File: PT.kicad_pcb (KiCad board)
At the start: 4 copper layers, 67 x 68 mm, 111 parts, among them J1 Conn_02x05_Odd_Even, J10 Conn_02x01, J11 Screw_Terminal_01x02, J2 USB_C_Receptacle_USB2.0_16P, J3 Conn_02x01, J4 Conn_02x01, J5 Screw_Terminal_01x05, J6 RJ45_Hanrun_HR911105A_Horizon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, J7 Conn_02x01, J8 Conn_02x01, J9 Conn_02x01, SW1 SKRPANE010, U1 USBLC6-2SC6, U2 STM32H563RIVx, U3 AP2112K-3.3, U4 TJA1042T-3, U5 LAN8742A, U6 ADS131A04, Y1 25 MHz, Y2 25 MHz, Y3 16.384 MHz

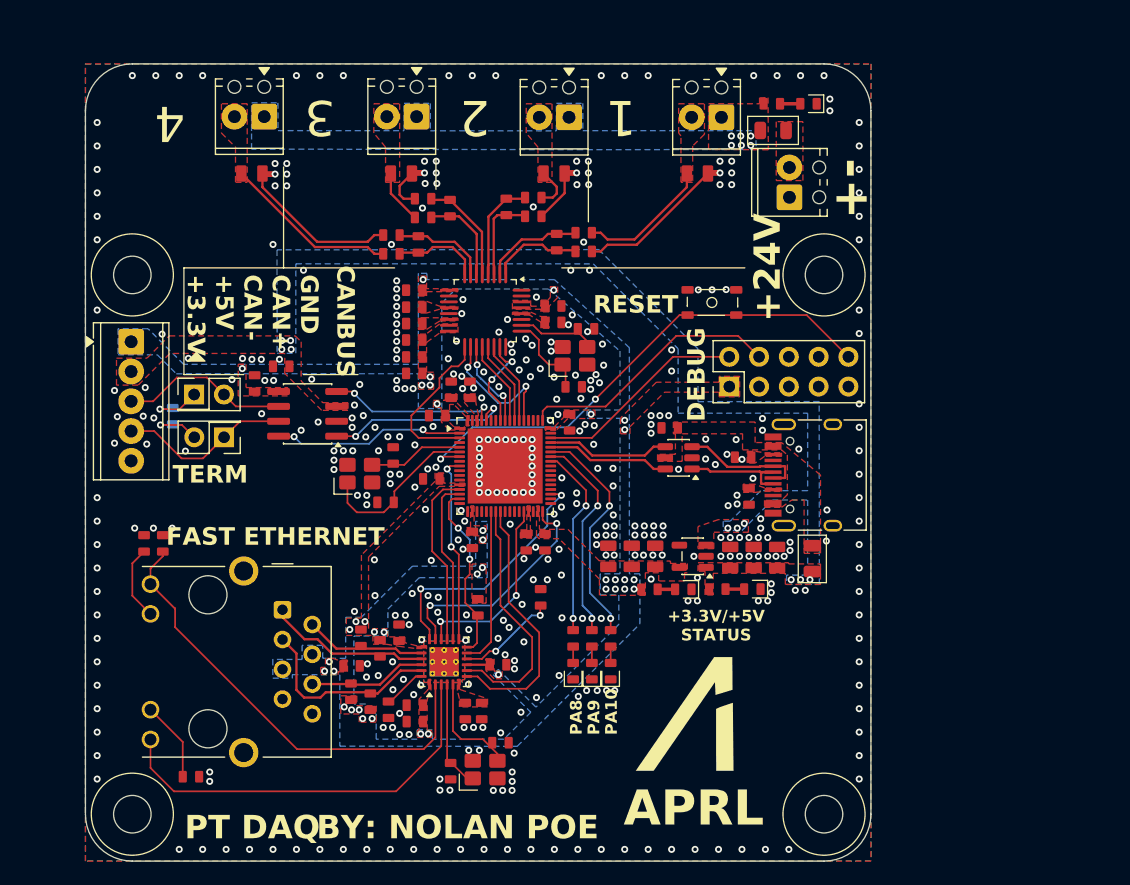
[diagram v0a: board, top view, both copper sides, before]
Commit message: holy hell 2 adcs
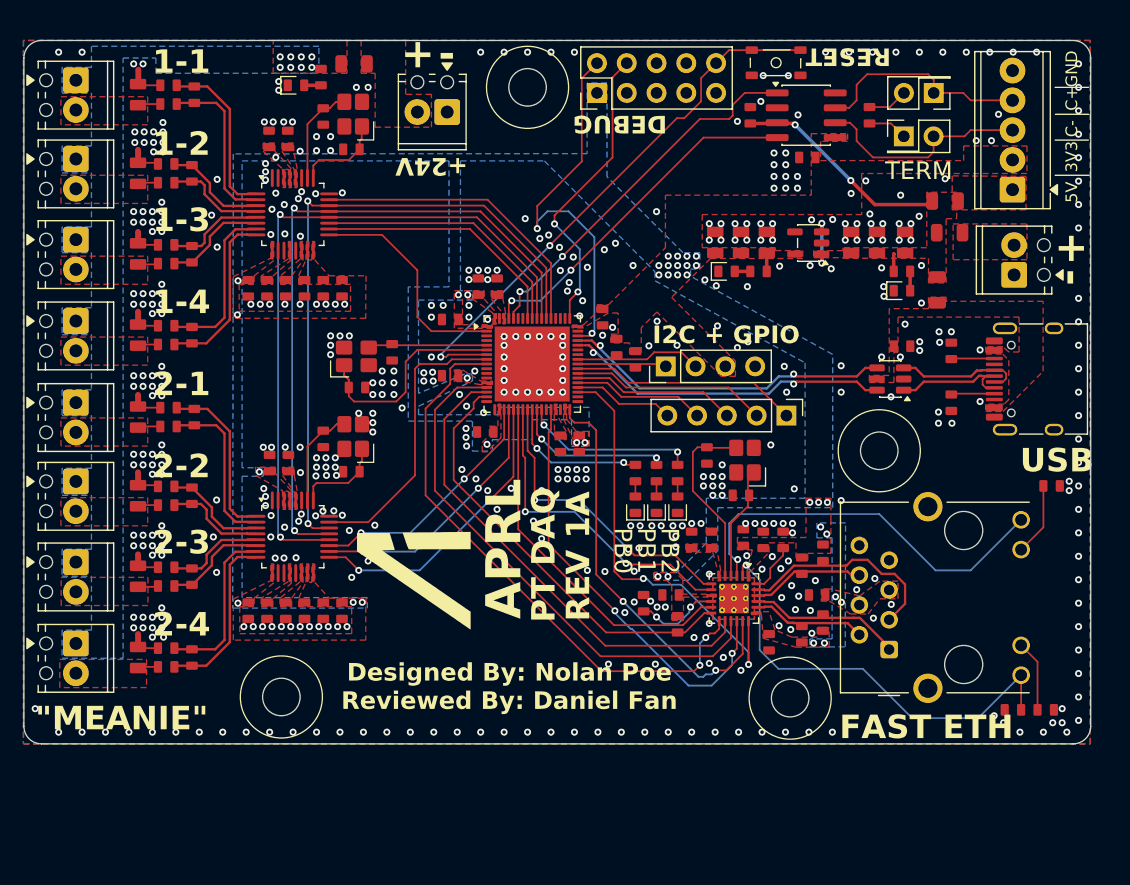
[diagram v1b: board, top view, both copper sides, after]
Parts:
- added C43: 10nF, APRLPrints:C_0603, F.Cu at (106.9, 103.5)
- added C44: 100nF, APRLPrints:C_0603, F.Cu at (111.5, 120.0)
- added C45: 100nF, APRLPrints:C_0603, F.Cu at (113.3, 107.4)
- added C46: 100nF, APRLPrints:C_0603, F.Cu at (116.3, 120.0)
- added C47: 100nF, APRLPrints:C_0603, F.Cu at (117.9, 120.0)
- added C48: 1uF, APRLPrints:C_0603, F.Cu at (119.5, 120.0)
- added C49: 1uF, APRLPrints:C_0603, F.Cu at (113.1, 120.0)
- added C50: 10nF, APRLPrints:C_0603, F.Cu at (106.7, 110.2)
- added C51: 1uF, APRLPrints:C_0603, F.Cu at (114.7, 120.0)
- added C52: 1uF, APRLPrints:C_0603, F.Cu at (114.9, 107.4)
- added C53: 10nF, APRLPrints:C_0603, F.Cu at (106.7, 117.1)
- added C54: 30pF, APRLPrints:C_0603, F.Cu at (117.9, 105.3)
- added C55: 30pF, APRLPrints:C_0603, F.Cu at (120.3, 108.1)
- added C56: 10nF, APRLPrints:C_0603, F.Cu at (106.7, 124.0)
- added F4: 100mA Hold, APRLPrints:Fuse_0805_2012Metric, F.Cu at (120.5, 73.3)
- added F5: 500mA, APRLPrints:Fuse_0805_2012Metric, F.Cu at (170.9, 85.0)
- added J12: Conn_01x04, Connector_PinHeader_2.54mm:PinHeader_1x04_P2.54mm_Vertical, F.Cu at (147.1, 99.1)
- added J13: Conn_02x01, TerminalBlock_Phoenix:TerminalBlock_Phoenix_MPT-0,5-2-2.54_1x02_P2.54mm_Horizontal, F.Cu at (96.8, 102.2)
- added J14: Conn_02x01, TerminalBlock_Phoenix:TerminalBlock_Phoenix_MPT-0,5-2-2.54_1x02_P2.54mm_Horizontal, F.Cu at (96.8, 108.9)
- added J15: Conn_02x01, TerminalBlock_Phoenix:TerminalBlock_Phoenix_MPT-0,5-2-2.54_1x02_P2.54mm_Horizontal, F.Cu at (96.8, 115.8)
- added J16: Conn_02x01, TerminalBlock_Phoenix:TerminalBlock_Phoenix_MPT-0,5-2-2.54_1x02_P2.54mm_Horizontal, F.Cu at (96.8, 122.8)
- added J17: Screw_Terminal_01x02, TerminalBlock_Phoenix:TerminalBlock_Phoenix_MPT-0,5-2-2.54_1x02_P2.54mm_Horizontal, F.Cu at (128.5, 77.4)
- added J18: Conn_01x05, Connector_PinHeader_2.54mm:PinHeader_1x05_P2.54mm_Vertical, F.Cu at (157.4, 103.3)
- added NT5: NetTie_2, NetTie:NetTie-2_SMD_Pad0.5mm, F.Cu at (102.1, 102.1)
- added NT6: NetTie_2, NetTie:NetTie-2_SMD_Pad0.5mm, F.Cu at (102.1, 108.7)
- added NT7: NetTie_2, NetTie:NetTie-2_SMD_Pad0.5mm, F.Cu at (102.1, 115.7)
- added NT8: NetTie_2, NetTie:NetTie-2_SMD_Pad0.5mm, F.Cu at (102.1, 122.5)
- added R32: 100R, APRLPrints:R_0603, F.Cu at (104.7, 104.2)
- added R33: 100R, APRLPrints:R_0805, F.Cu at (102.1, 103.5)
- added R34: 100R, APRLPrints:R_0603, F.Cu at (104.7, 102.7)
- added R35: 100R, APRLPrints:R_0603, F.Cu at (104.5, 111.0)
- added R36: 100R, APRLPrints:R_0805, F.Cu at (102.1, 110.2)
- added R37: 100R, APRLPrints:R_0603, F.Cu at (104.5, 109.4)
- added R38: 100R, APRLPrints:R_0603, F.Cu at (104.5, 117.9)
- added R39: 100R, APRLPrints:R_0805, F.Cu at (102.1, 117.0)
- added R40: 100R, APRLPrints:R_0603, F.Cu at (104.5, 116.3)
- added R41: 100R, APRLPrints:R_0603, F.Cu at (104.5, 124.8)
- added R42: 100R, APRLPrints:R_0805, F.Cu at (102.1, 124.0)
- added R43: 100R, APRLPrints:R_0603, F.Cu at (104.5, 123.2)
- added R44: 10k, APRLPrints:R_0603, F.Cu at (144.5, 98.5)
- added R45: 10k, APRLPrints:R_0603, F.Cu at (142.9, 97.5)
- added U7: ADS131A04, libpt:QFP-32_5x5_Pitch0.5mm, F.Cu at (115.3, 113.7)
- added Y4: 16.384 MHz, APRLPrints:3225-4P-L, F.Cu at (120.5, 105.1)
- F2: value 100mA Hold -> 500mA
- J11: value Screw_Terminal_01x02 -> Conn_02x01
- J3: value Conn_02x01 -> Screw_Terminal_01x02; footprint Connector_PinHeader_2.54mm:PinHeader_2x01_P2.54mm_Vertical -> TerminalBlock_Phoenix:TerminalBlock_Phoenix_MPT-0,5-2-2.54_1x02_P2.54mm_Horizontal
- J5: value Screw_Terminal_01x05 -> Conn_02x01; footprint TerminalBlock_Phoenix:TerminalBlock_Phoenix_MPT-0,5-5-2.54_1x05_P2.54mm_Horizontal -> Connector_PinHeader_2.54mm:PinHeader_2x01_P2.54mm_Vertical
- J6: value RJ45_Hanrun_HR911105A_Horizontal -> Screw_Terminal_01x05; footprint Connector_RJ:RJ45_Hanrun_HR911105A_Horizontal -> TerminalBlock_Phoenix:TerminalBlock_Phoenix_MPT-0,5-5-2.54_1x05_P2.54mm_Horizontal
- J7: value Conn_02x01 -> RJ45_Hanrun_HR911105A_Horizontal; footprint TerminalBlock_Phoenix:TerminalBlock_Phoenix_MPT-0,5-2-2.54_1x02_P2.54mm_Horizontal -> Connector_RJ:RJ45_Hanrun_HR911105A_Horizontal
- R9: moved to F.Cu
- moved R19 78.2 mm to (179.5, 128.4), turned to 0 degrees
- moved R18 77.5 mm to (180.0, 109.3)
- moved R17 73.9 mm to (176.7, 128.4), turned to 180 degrees
- moved J6 71.8 mm to (176.7, 84.1), turned to 90 degrees
- moved H2 70.6 mm to (135.3, 75.3)
- moved J3 68.8 mm to (176.8, 91.3), turned to 90 degrees
- moved J5 68.2 mm to (167.4, 79.5), turned to 0 degrees
- moved J4 68.1 mm to (170.0, 75.8), turned to 180 degrees
- moved R9 64.7 mm to (164.5, 77.7), turned to -90 degrees
- moved J11 61.8 mm to (96.8, 95.3), turned to -90 degrees
- moved C25 50.9 mm to (159.2, 81.3), turned to 180 degrees
- moved NT1 49.8 mm to (102.1, 74.3), turned to -90 degrees
- moved U4 49.6 mm to (159.1, 77.7), turned to 0 degrees
- moved R21 48.2 mm to (102.1, 76.0), turned to 90 degrees
- moved J7 47.6 mm to (166.2, 123.3), turned to 90 degrees
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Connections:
- net /Analog/AIN1+ renamed /ADC 1/AIN1+
- net /Analog/AIN1- renamed /ADC 1/AIN1-
- net /Analog/AIN1_SENSE- renamed /ADC 1/AIN1_SENSE-
- net /Analog/AIN2+ renamed /ADC 1/AIN2+
- net /Analog/AIN2- renamed /ADC 1/AIN2-
- net /Analog/AIN2_SENSE- renamed /ADC 1/AIN2_SENSE-
- net /Analog/AIN3+ renamed /ADC 1/AIN3+
- net /Analog/AIN3- renamed /ADC 1/AIN3-
- net /Analog/AIN3_SENSE- renamed /ADC 1/AIN3_SENSE-
- net /Analog/AIN4+ renamed /ADC 1/AIN4+
- net /Analog/AIN4- renamed /ADC 1/AIN4-
- net /Analog/AIN4_SENSE- renamed /ADC 1/AIN4_SENSE-
- net /Analog/MISO renamed /ADC 1/MISO
- net /Analog/MOSI renamed /ADC 1/MOSI
- net /Analog/SCLK renamed /ADC 1/SCLK
- net /Analog/~{DRDY} renamed /ADC 1/~{DRDY}
- F2 pad 1: +24V -> Net-(J3-Pin_2)
- F2 pad 2: Net-(J11-Pin_2) -> +5V
- J10 pad 2: /Analog/AIN4_SENSE+ -> /ADC 1/AIN3_SENSE+
- J11 pad 1: GND -> +24V
- J11 pad 2: Net-(J11-Pin_2) -> /ADC 1/AIN4_SENSE+
- J3 pad 1: /Connectivity/CAN+ -> GND
- J4 pad 1: Net-(J4-Pin_1) -> /Connectivity/CAN+
- J4 pad 2: /Connectivity/CAN- -> Net-(J4-Pin_2)
- J5 pad 1: +3.3V -> Net-(J5-Pin_1)
- J5 pad 2: +5V -> /Connectivity/CAN-
- J6 pad 1: /Connectivity/TX+ -> Net-(J6-Pin_1)
- J6 pad 2: /Connectivity/TX- -> +3.3V
- J6 pad 3: /Connectivity/RX+ -> /Connectivity/CAN-
- J6 pad 4: +3.3V -> /Connectivity/CAN+
- J6 pad 5: +3.3V -> GND
- J7 pad 1: +24V -> /Connectivity/TX+
- J7 pad 2: /Analog/AIN1_SENSE+ -> /Connectivity/TX-
- J8 pad 2: /Analog/AIN2_SENSE+ -> /ADC 1/AIN1_SENSE+
- J9 pad 2: /Analog/AIN3_SENSE+ -> /ADC 1/AIN2_SENSE+
- R18 pad 1: Net-(J6-Pad11) -> Net-(J7-Pad11)
- R19 pad 1: Net-(J6-Pad10) -> Net-(J7-Pad10)
- R20 pad 1: /Analog/AIN1_SENSE+ -> /ADC 1/AIN1_SENSE+
- R21 pad 1: /Analog/AIN1_SENSE+ -> /ADC 1/AIN1_SENSE+
- R23 pad 1: /Analog/AIN2_SENSE+ -> /ADC 1/AIN2_SENSE+
- R24 pad 1: /Analog/AIN2_SENSE+ -> /ADC 1/AIN2_SENSE+
- R26 pad 1: /Analog/AIN3_SENSE+ -> /ADC 1/AIN3_SENSE+
- R27 pad 1: /Analog/AIN3_SENSE+ -> /ADC 1/AIN3_SENSE+
- R29 pad 1: /Analog/AIN4_SENSE+ -> /ADC 1/AIN4_SENSE+
- R30 pad 1: /Analog/AIN4_SENSE+ -> /ADC 1/AIN4_SENSE+
- R9 pad 1: Net-(J3-Pin_2) -> Net-(J4-Pin_2)
- R9 pad 2: Net-(J4-Pin_1) -> Net-(J5-Pin_1)
- U2 pad 2: /Connectivity/FDCAN_STDBY -> /ADC 1/~{ADC_RESET}
- U2 pad 20: unconnected-(U2-PA4-Pad20) -> /ADC 2/~{DRDY}
- U2 pad 21: unconnected-(U2-PA5-Pad21) -> /ADC 2/~{DONE}
- U2 pad 22: unconnected-(U2-PA6-Pad22) -> /ADC 2/~{ADC_RESET}
- U2 pad 26: unconnected-(U2-PB0-Pad26) -> /Microcontroller/USER_LED_1
- U2 pad 27: unconnected-(U2-PB1-Pad27) -> /Microcontroller/USER_LED_2
- U2 pad 28: unconnected-(U2-PB2-Pad28) -> /Microcontroller/USER_LED_3
- U2 pad 3: /Analog/~{ADC_RESET} -> unconnected-(U2-PC14-Pad3)
- U2 pad 38: unconnected-(U2-PD11-Pad38) -> /Microcontroller/GPIO5
- U2 pad 39: unconnected-(U2-PD12-Pad39) -> /Microcontroller/GPIO4
- U2 pad 40: unconnected-(U2-PC6-Pad40) -> /Microcontroller/GPIO3
- U2 pad 41: unconnected-(U2-PC7-Pad41) -> /Microcontroller/GPIO2
- U2 pad 42: unconnected-(U2-PC8-Pad42) -> /Microcontroller/GPIO1
- U2 pad 43: unconnected-(U2-PC9-Pad43) -> /Microcontroller/I2C_SDA
- U2 pad 44: /Microcontroller/USER_LED_1 -> /Microcontroller/I2C_SCL
- U2 pad 45: /Microcontroller/USER_LED_2 -> unconnected-(U2-PA9-Pad45)
- U2 pad 46: /Microcontroller/USER_LED_3 -> unconnected-(U2-PA10-Pad46)
- U2 pad 56: /Analog/~{DONE} -> /ADC 1/~{CS}
- U2 pad 61: /Analog/~{CS} -> /ADC 1/~{DONE}
- U2 pad 8: unconnected-(U2-PC0-Pad8) -> /ADC 2/~{CS}
- U6 pad 17: /Analog/~{ADC_RESET} -> /ADC 1/~{ADC_RESET}
- U6 pad 18: /Analog/~{DONE} -> /ADC 1/~{DONE}
- U6 pad 23: /Analog/~{CS} -> /ADC 1/~{CS}
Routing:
- net /ADC 1/MOSI: track 7.24 -> 59.6 mm, vias 0 -> 2
- net /ADC 1/MISO: track 7.19 -> 58.1 mm, vias 0 -> 2
- net /ADC 1/SCLK: track 7.15 -> 56.5 mm, vias 0 -> 2
- net /Connectivity/ETH_MDC: track 16.1 -> 49.4 mm
- net /Connectivity/ETH_~{RST}: track 15.1 -> 45.3 mm
- net /Connectivity/ETH_REF_CLK: track 14.1 -> 41.2 mm
- net /ADC 1/~{CS}: track 0.00 -> 25.9 mm
- net /ADC 2/~{ADC_RESET}: track 0.00 -> 25.2 mm, vias 0 -> 2
- net /ADC 2/~{CS}: track 0.00 -> 24.5 mm
- net +5V: track 0.00 -> 24.5 mm, vias 10 -> 4
- net /ADC 2/~{DONE}: track 0.00 -> 22.8 mm, vias 0 -> 2
- net /ADC 1/~{DONE}: track 0.00 -> 21.7 mm
- net /Connectivity/ETH_MDIO: track 15.3 -> 36.7 mm, vias 2 -> 0
- net /ADC 2/~{DRDY}: track 0.00 -> 21.2 mm, vias 0 -> 2
- net /Connectivity/ETH_TX_EN: track 16.4 -> 37.2 mm
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- added copper zone on F.Cu, net (none)
- added copper zone on F.Cu, net /ADC 1/AIN1_SENSE+
- added copper zone on F.Cu, net /ADC 1/AIN2_SENSE+
- added copper zone on F.Cu, net /ADC 1/AIN3_SENSE+
- added copper zone on F.Cu, net /ADC 1/AIN4_SENSE+
- added copper zone on F.Cu, net /ADC 2/AIN1_SENSE+
- added copper zone on F.Cu, net /ADC 2/AIN2_SENSE+
- added copper zone on F.Cu, net /ADC 2/AIN3_SENSE+
- added copper zone on F.Cu, net /ADC 2/AIN4_SENSE+
- added copper zone on F.Cu, net /Microcontroller/+24_IN
- added copper zone on F.Cu, net Net-(J3-Pin_2)
- added copper zone on F.Cu, net Net-(U7-CAP)
- added copper zone on F.Cu, net Net-(U7-REFEXT)
- added copper zone on F.Cu, net Net-(U7-REFP)
- removed copper zone on B.Cu, net +5V
- removed copper zone on F.Cu, net /Analog/AIN1_SENSE+
- removed copper zone on F.Cu, net /Analog/AIN2_SENSE+
- removed copper zone on F.Cu, net /Analog/AIN3_SENSE+
- removed copper zone on F.Cu, net /Analog/AIN4_SENSE+
- removed copper zone on F.Cu, net Net-(J11-Pin_2)
- removed copper zone on F.Cu, net Net-(J2-CC1)
- removed copper zone on F.Cu, net Net-(J2-CC2)
- removed copper zone on F.Cu, net Net-(U5-VDDCR)
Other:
- board size 67 x 68 mm -> 91 x 60 mm
- board text added: "1-1"
- board text added: "1-2"
- board text added: "1-3"
- board text added: "1-4"
- board text added: "2-1"
- board text added: "2-2"
- board text added: "2-3"
- board text added: "2-4"
- board text added: "3V3"
- board text added: "5V"
- board text added: "C+"
- board text added: "C-"
- board text added: "Designed By: Nolan Poe Reviewed By: Daniel Fan"
- board text added: "FAST ETH"
- board text added: "GND"
- board text added: "I2C + GPIO"
- board text added: "PB0"
- board text added: "PB1"
- board text added: "PB2"
- board text added: "REV 1A"
- board text added: "USB"
- board text added: "{dblquote}MEANIE{dblquote}"
- board text removed: "+3.3V/+5V STATUS"
- board text removed: "1"
- board text removed: "2"
- board text removed: "3"
- board text removed: "4"
- board text removed: "BY: NOLAN POE"
- board text removed: "CANBUS"
- board text removed: "FAST ETHERNET"
- board text removed: "GND CAN+ CAN- +5V +3.3V"
- board text removed: "PA10"
- board text removed: "PA8"
- board text removed: "PA9"
- board text removed: "UNDER NORMAL OPERATION, ONLY USE INTERAL +3.3V EXTERNAL +3.3V IS UNFUSED AND UNFILTERED AND BACKFLOWS TO +5V"
